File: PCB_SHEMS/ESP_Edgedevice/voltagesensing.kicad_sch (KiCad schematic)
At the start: 36 parts, among them J4 Conn_01x02, U3 AMS1117-5.0, U4 AMC1200SDUBR, U5 OPA333xxDBV, U6 OPA333xxDBV, U7 MCP3202

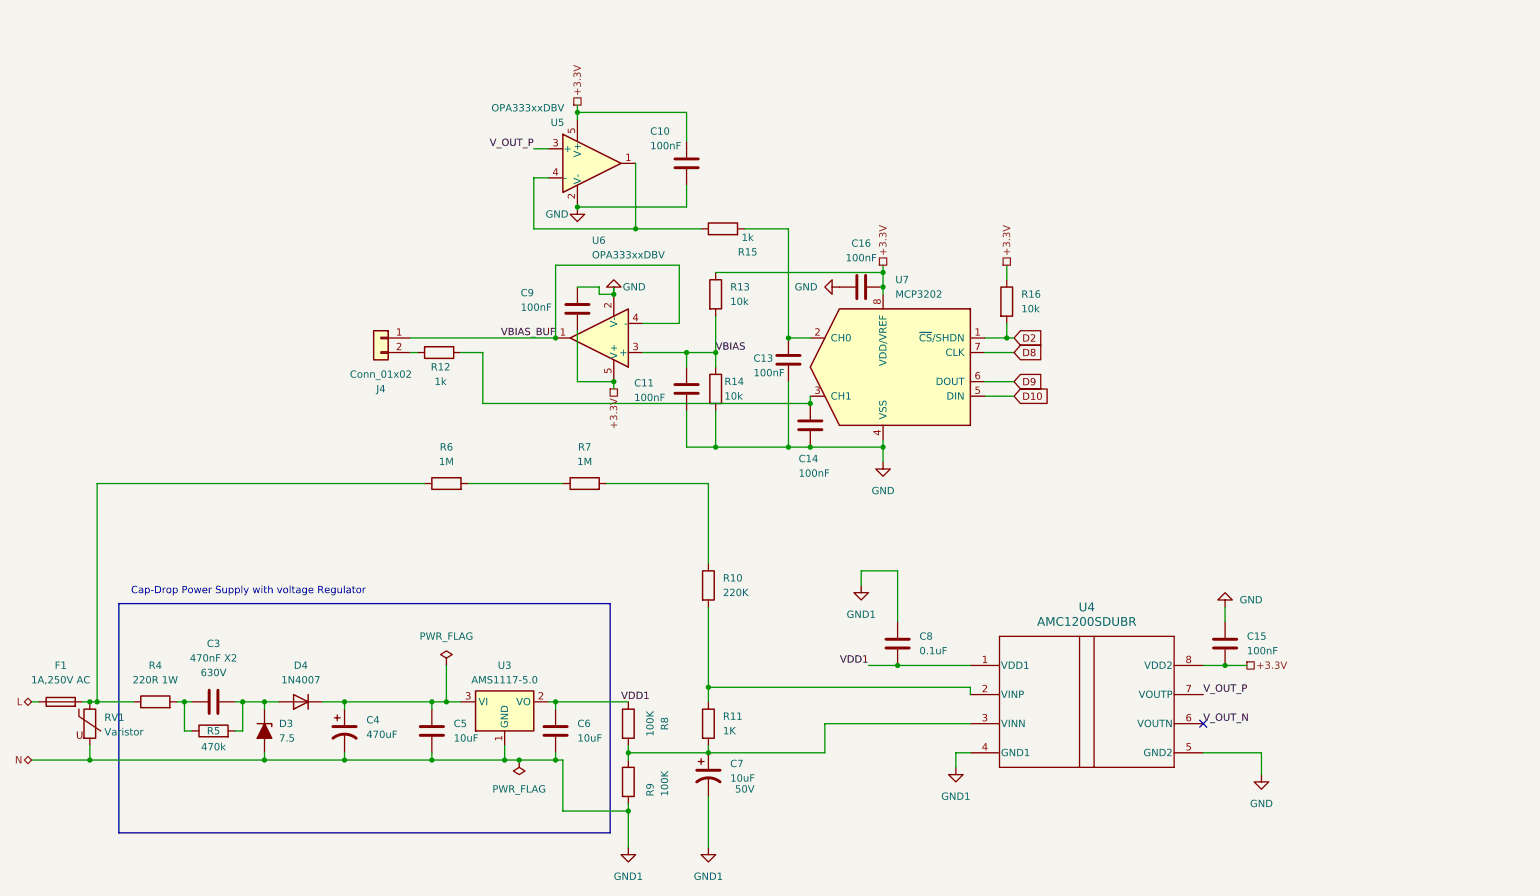
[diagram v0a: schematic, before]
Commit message: 2nd ADS
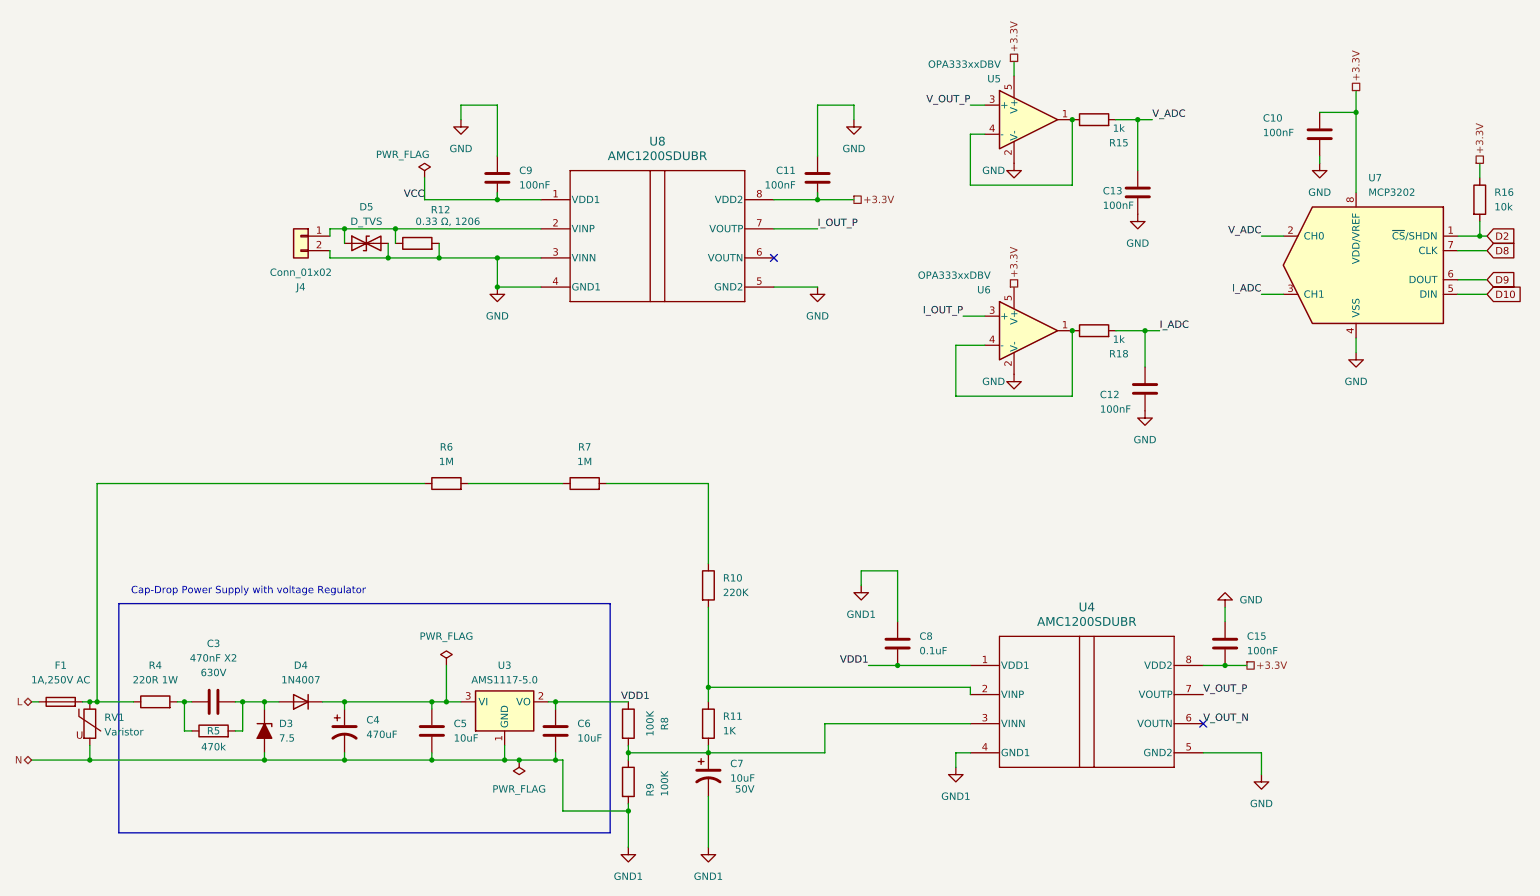
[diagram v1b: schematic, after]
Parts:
- removed C14, C16: 100nF, Capacitor_SMD:C_1206_3216Metric, symbol Device:C
- removed R13, R14: 10k, Resistor_SMD:R_1206_3216Metric, symbol Device:R
- added C12: 100nF, Capacitor_SMD:C_1206_3216Metric, symbol Device:C
- added D5: D_TVS, Diode_SMD:Nexperia_DSN0603-2_0.6x0.3mm_P0.4mm, symbol Device:D_TVS
- added R18: 1k, Resistor_SMD:R_1206_3216Metric, symbol Device:R
- added U8: AMC1200SDUBR, AMC1200SDUBR:DUB0008A-IPC_A, symbol 2025-08-05_00-17-59:AMC1200SDUBR
- R12: value 1k -> 0.33 Ω, 1206
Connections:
- net +3.3V: now also C11.2, U8.8 (VDD2); no longer C9.1
- net GND: now also C11.1, C9.1, J4.2 (Pin_2), R12.2, C12.1, D5.2 (A2), U8.3 (VINN), U8.4 (GND1), U8.5 (GND2); no longer C11.2, C9.2
- net V_ADC: now reaches C13.1, R15.2, U7.2 (CH0)
- net at R12.1: now also J4.1 (Pin_1), D5.1 (A1), U8.2 (VINP); no longer U7.3 (CH1)
- net VBIAS renamed I_OUT_P
- net I_OUT_P: now also U8.7 (VOUTP); no longer C11.1
- net VBIAS_BUF: no longer names the net of U6.1, U6.4 (-)
- net VBIAS_BUF: now also R18.1; no longer J4.1 (Pin_1)
- new net I_ADC: C12.2, R18.2, U7.3 (CH1)
- new net VCC: C9.2, U8.1 (VDD1)
- no-connect marks 1 -> 2
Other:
- moved on the sheet: J4, R15, R16, U5
